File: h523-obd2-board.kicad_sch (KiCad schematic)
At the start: 68 parts, among them J1 Conn_02x05_Odd_Even, J2 Conn_01x03, J3 Conn_01x03, J4 Conn_01x03, J5 Conn_01x03, J6 Conn_01x03, J7 Conn_01x03, J8 Conn_01x03, J9 Conn_01x03, Q1 AO3400A, U1 STM32H523CEUx, U2 HT7533-1-SOT89, U3 SN65HVD230, U5 ADXL345, Y1 Crystal_25MHz

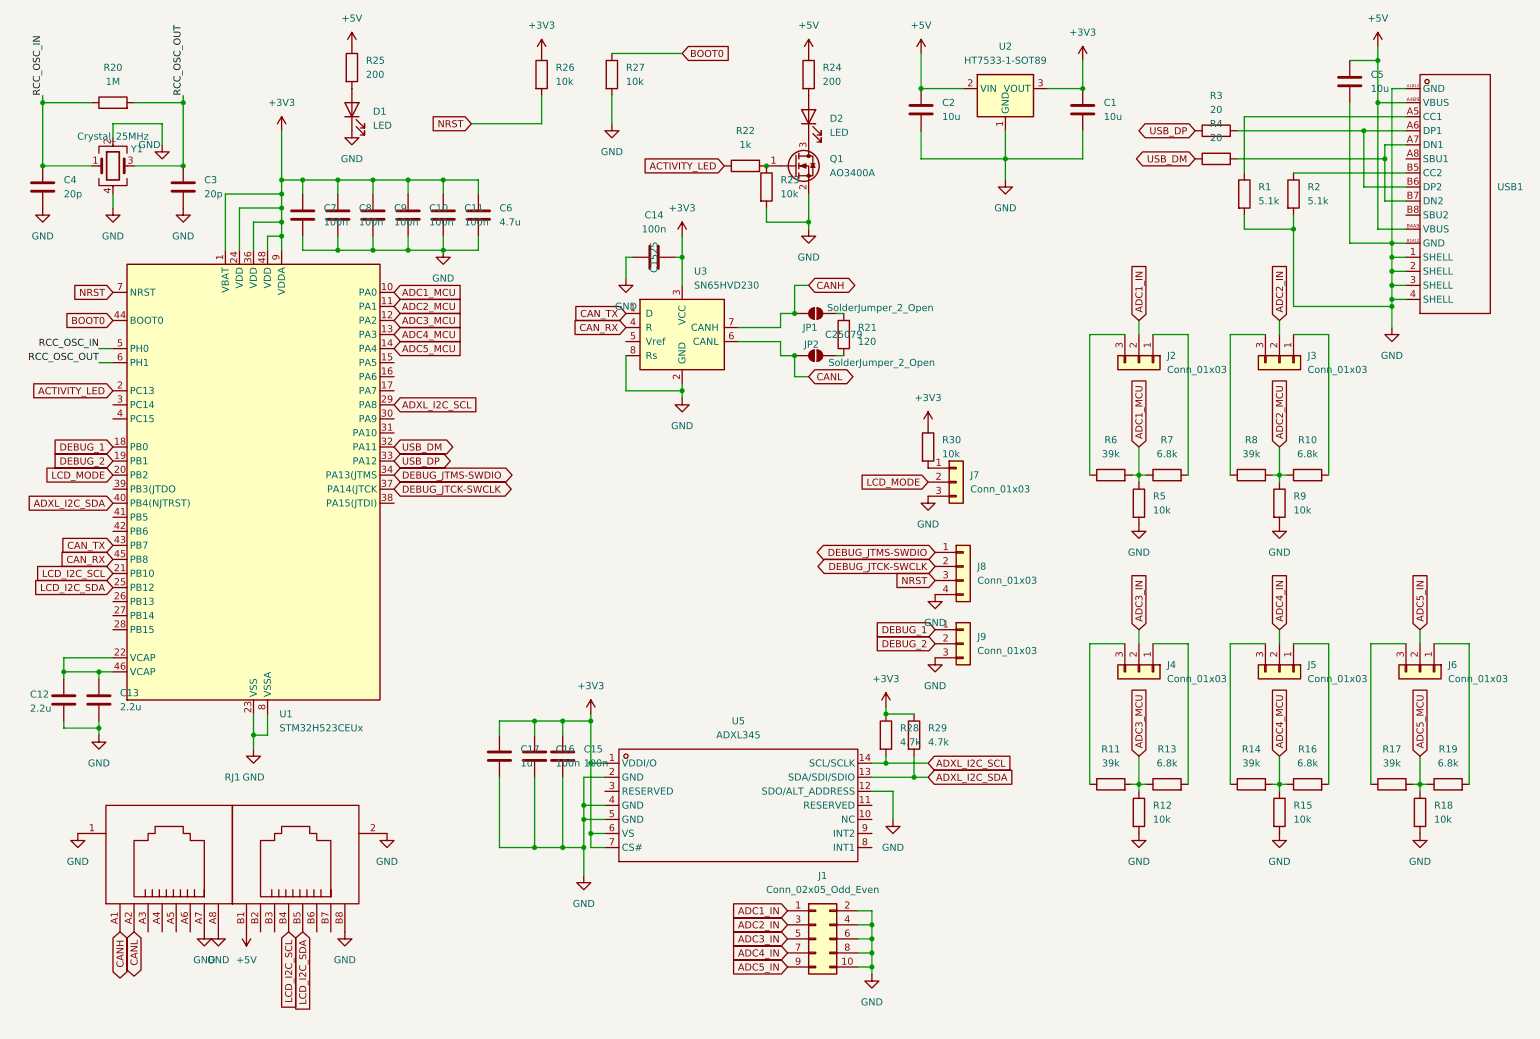
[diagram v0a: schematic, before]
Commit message: PROTO A manufactured
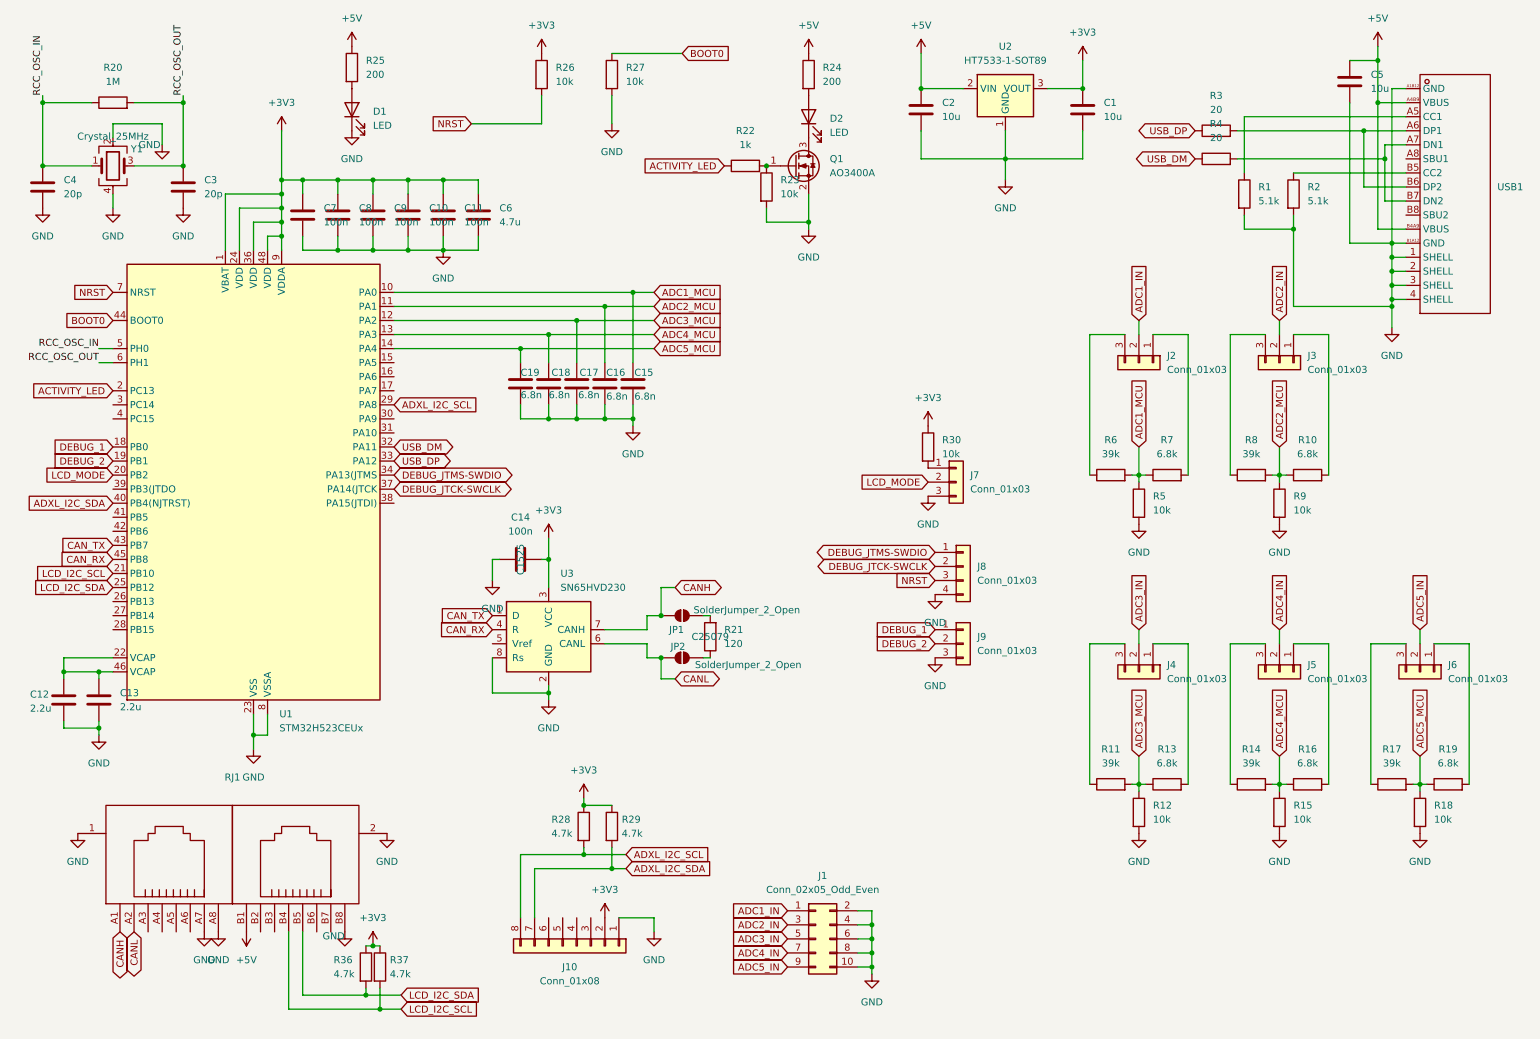
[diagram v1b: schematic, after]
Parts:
- removed U5: ADXL345, JLCLibrary:ADXL345, symbol JLCLibrary:ADXL345BCCZ-RL
- added C18, C19: 6.8n, Capacitor_SMD:C_0402_1005Metric, symbol Device:C
- added J10: Conn_01x08, Connector_PinHeader_2.54mm:PinHeader_1x08_P2.54mm_Vertical, symbol Connector_Generic:Conn_01x08
- added R36, R37: 4.7k, Resistor_SMD:R_0402_1005Metric, symbol Device:R
- C12, C13: LCSC C12530 -> C23630
- C15, C16: value 100n -> 6.8n; LCSC C1525 -> C1542
- C17: value 1u -> 6.8n; footprint Capacitor_SMD:C_0603_1608Metric -> Capacitor_SMD:C_0402_1005Metric; LCSC C15849 -> C1542
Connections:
- net +3V3: now also J10.2 (Pin_2), R36.1, R37.1; no longer C15.1, C16.1, C17.1
- net ADC1_MCU: now also C15.2
- net ADC2_MCU: now also C16.2
- net ADC3_MCU: now also C17.2
- net ADC4_MCU: now also C18.2
- net ADC5_MCU: now also C19.2
- net ADXL_I2C_SCL: now also J10.8 (Pin_8)
- net ADXL_I2C_SDA: now also J10.7 (Pin_7)
- net GND: now also C15.1, C16.1, C17.1, C18.1, C19.1, J10.1 (Pin_1); no longer C15.2, C16.2, C17.2
- net LCD_I2C_SCL: now also R37.2
- net LCD_I2C_SDA: now also R36.2
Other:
- moved on the sheet: C14, JP1, JP2, R21, R28, R29, U3
